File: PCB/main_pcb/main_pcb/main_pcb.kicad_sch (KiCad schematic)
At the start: 50 parts, among them J1 Conn_01x20_Socket, J2 Conn_01x20_Socket, SW0_Header1 B6B-XH-A, SW1_Header1 B6B-XH-A

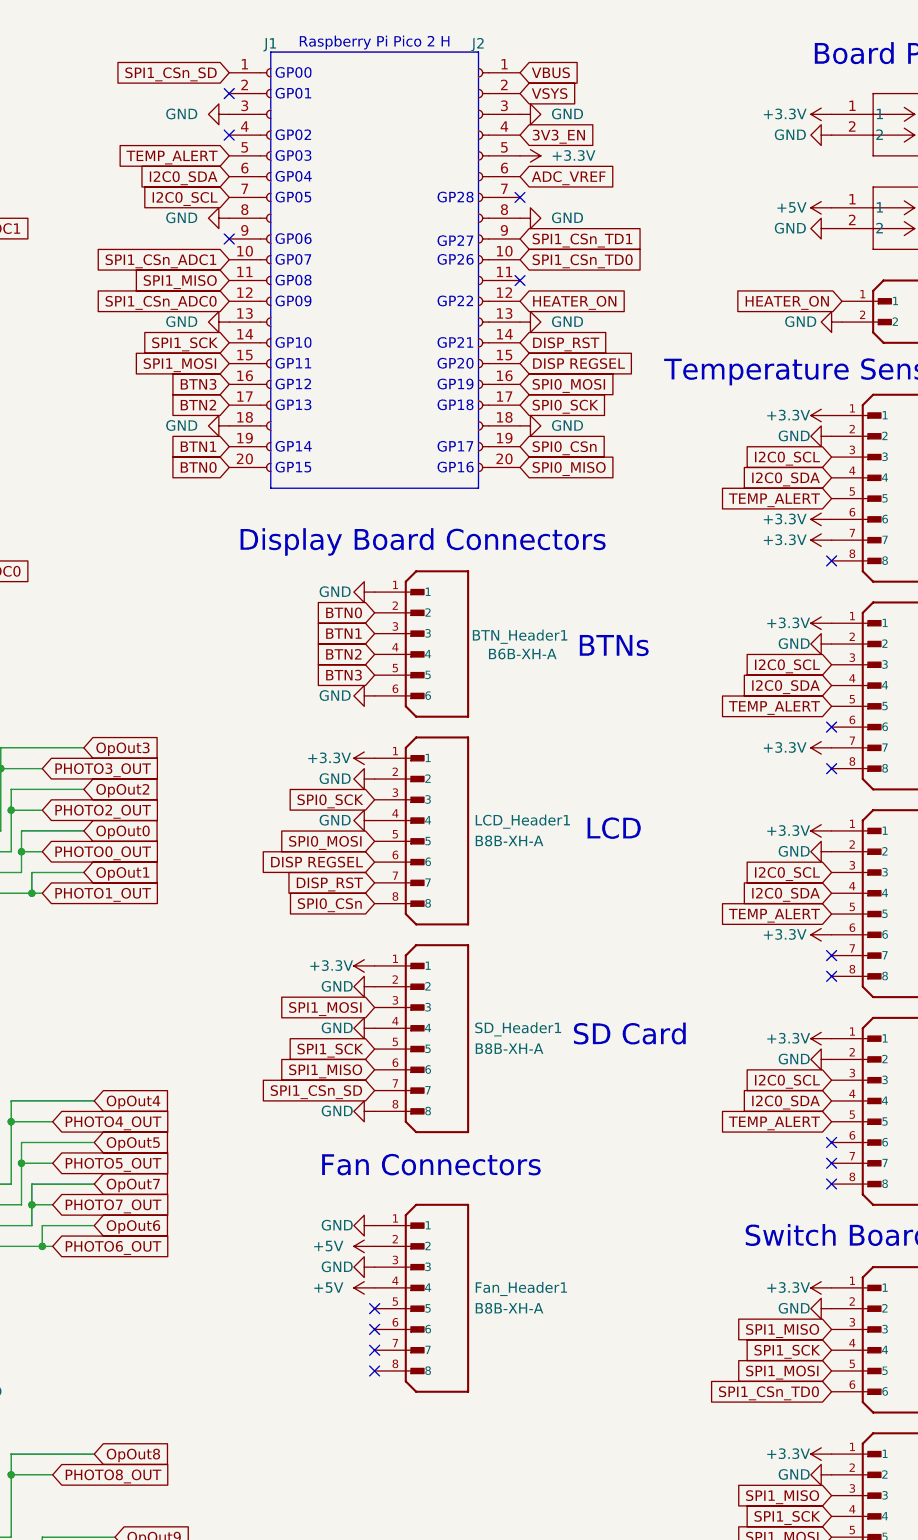
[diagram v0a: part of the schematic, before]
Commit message: Fixed some stuff and made the main PCB smaller.
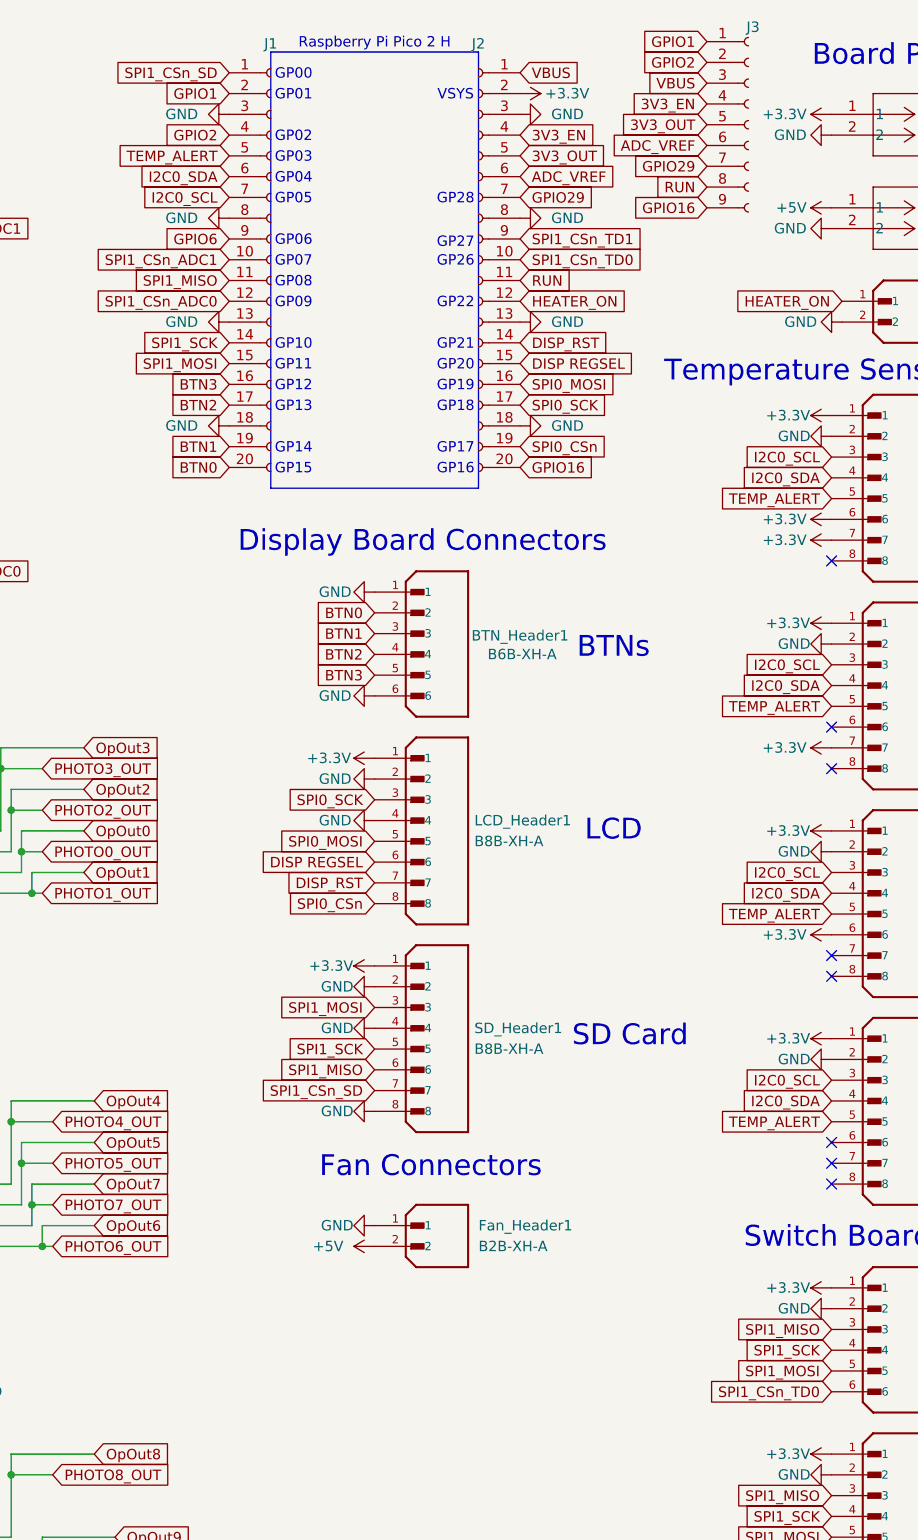
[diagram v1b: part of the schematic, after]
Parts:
- removed Fan_Header1: B8B-XH-A, Connector_JST:JST_XH_B8B-XH-A_1x08_P2.50mm_Vertical, symbol B8B-XH-A:B8B-XH-A
- added Fan_Header1: B2B-XH-A, B2B_XH_A:JST_B2B-XH-A, symbol B2B-XH-A:B2B-XH-A
- added J3: Conn_01x09_Socket, Connector_PinSocket_2.54mm:PinSocket_1x09_P2.54mm_Vertical, symbol Connector:Conn_01x09_Socket
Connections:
- net VSYS is gone; now on net +3.3V: J2.2 (Pin_2)
- net +3.3V: no longer J2.5 (Pin_5)
- net +5V: now also Fan_Header1.2
- net 3V3_EN: now also J3.4 (Pin_4)
- net ADC_VREF: now also J3.6 (Pin_6)
- net GND: now also Fan_Header1.1
- net VBUS: now also J3.3 (Pin_3)
- net RUN: now reaches J2.11 (Pin_11)
- net RUN: now also J3.8 (Pin_8)
- net GPIO29: now reaches J2.7 (Pin_7)
- net GPIO29: now also J3.7 (Pin_7)
- net GPIO1: now reaches J1.2 (Pin_2)
- net GPIO1: now also J3.1 (Pin_1)
- net GPIO2: now reaches J1.4 (Pin_4)
- net GPIO2: now also J3.2 (Pin_2)
- net GPIO6: now reaches J1.9 (Pin_9)
- net SPI0_MISO renamed GPIO16
- net GPIO16: now also J3.9 (Pin_9)
- new net 3V3_OUT: J2.5 (Pin_5), J3.5 (Pin_5)
- no-connect marks 27 -> 18
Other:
- note added: "VSYS"
